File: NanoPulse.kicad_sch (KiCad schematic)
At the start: 0 parts

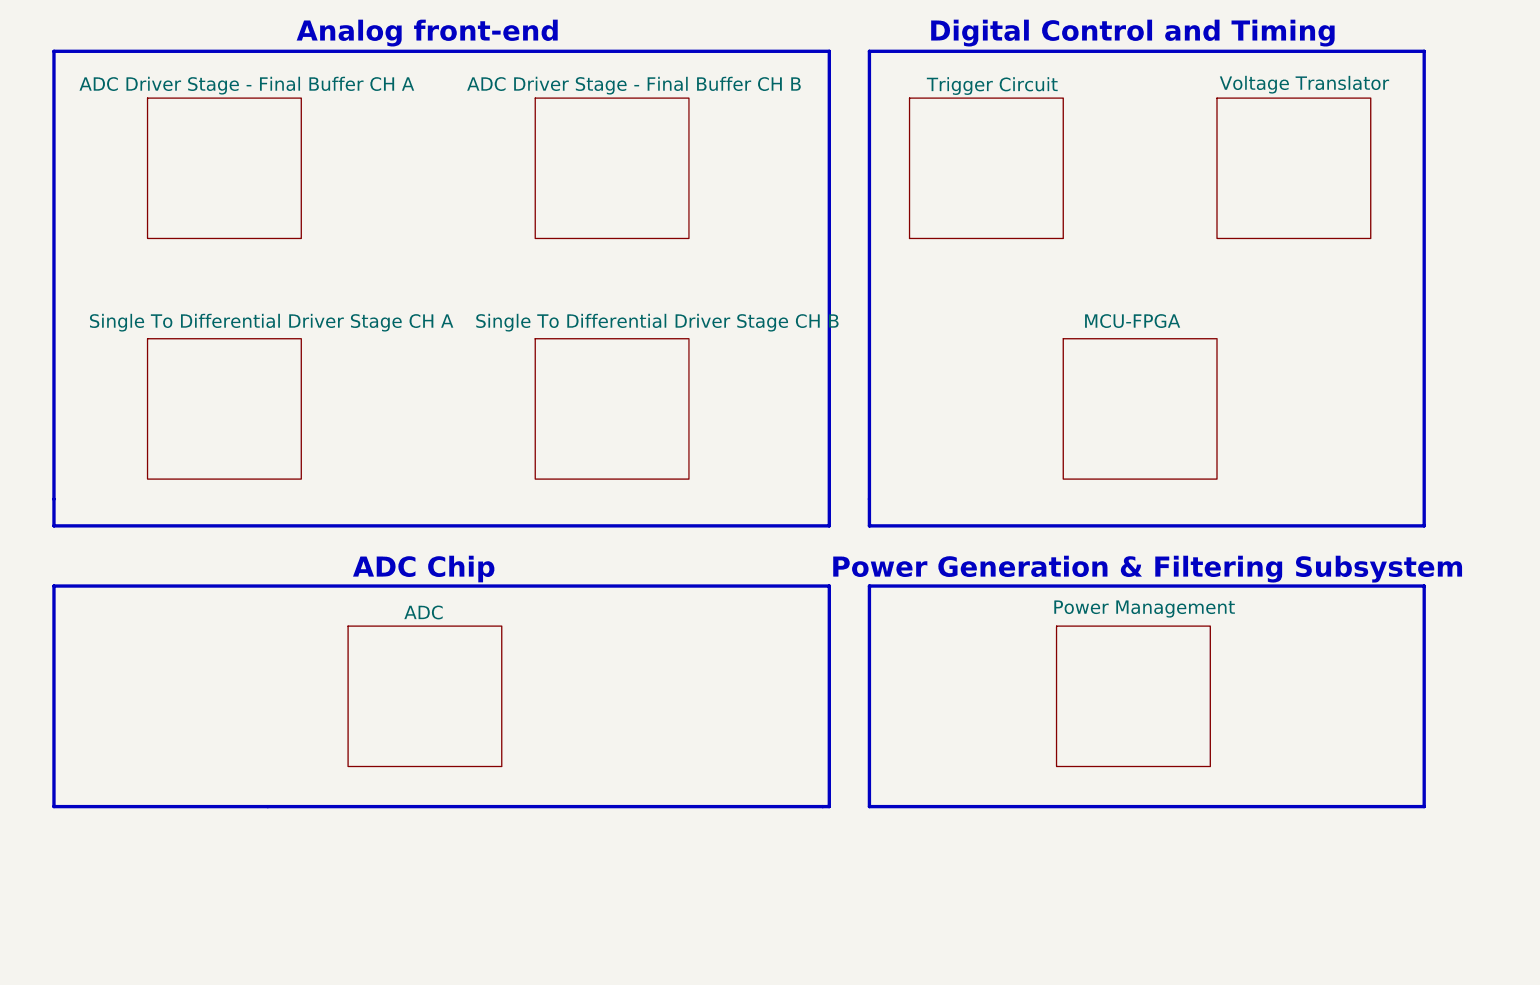
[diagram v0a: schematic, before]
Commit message: All done, Gerberd out :)
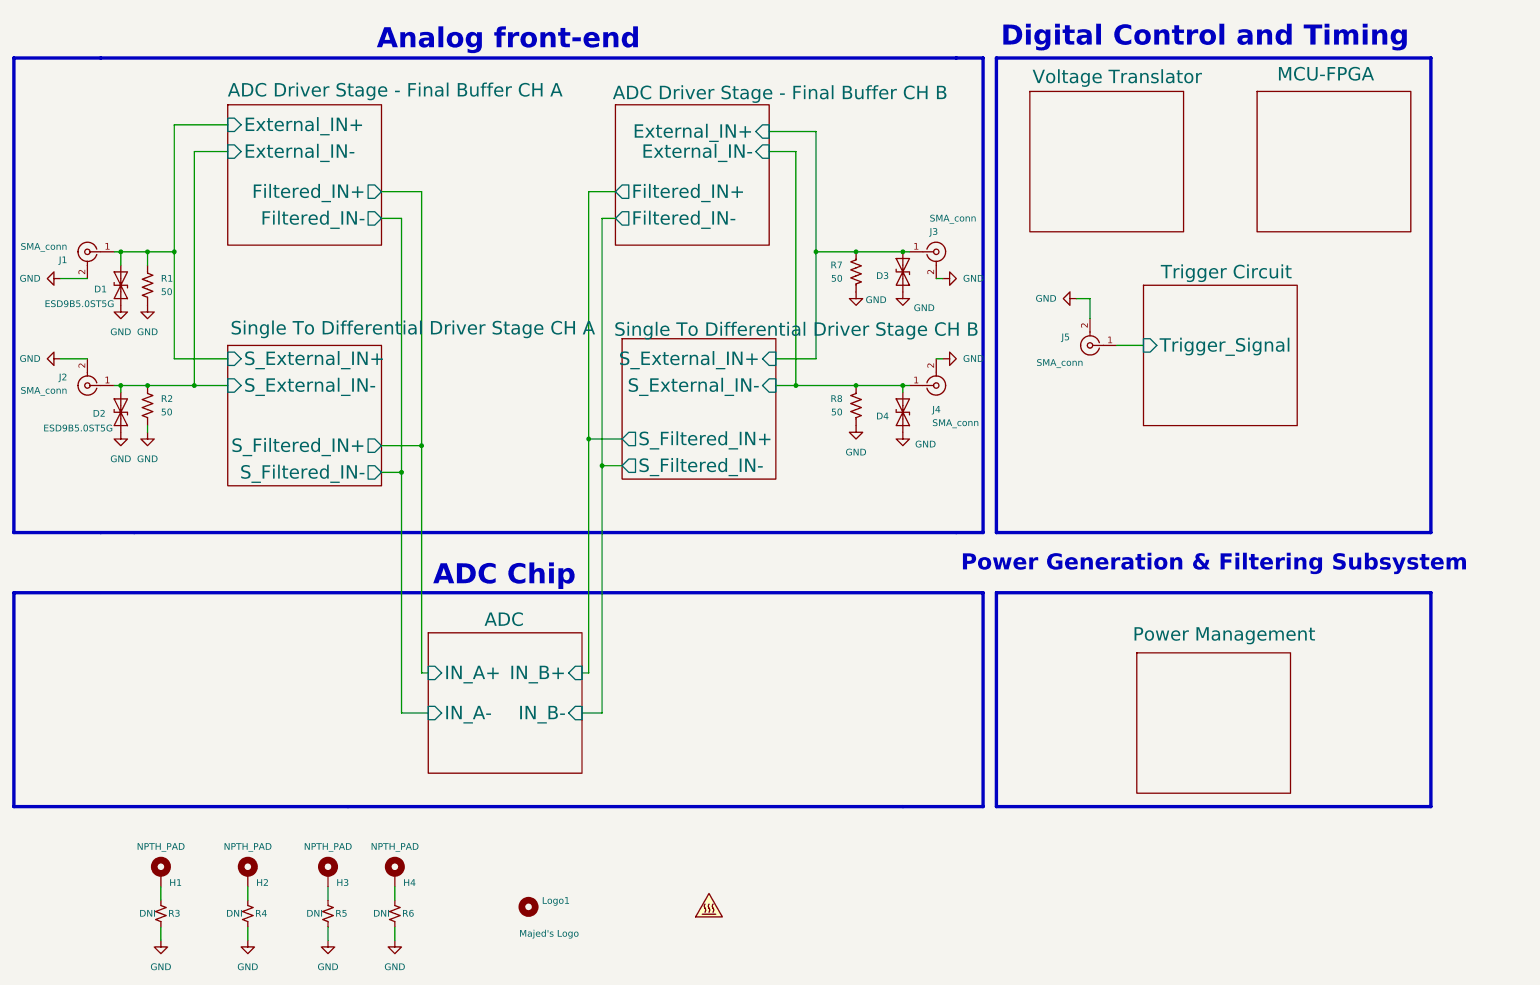
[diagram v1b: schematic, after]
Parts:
- added D1, D2, D3, D4: ESD9B5.0ST5G, Diode_SMD:D_SOD-923, symbol majed-symbols:ESD9B5.0ST5G
- added H1, H2, H3, H4: NPTH_PAD, Mounting_Wuerth:Mounting_Wuerth_WA-SMSI-M1.6_H3.5mm_ThreadDepth2mm_NoNPTH_97730356330, symbol majed-symbols:MountingHole_Pad_1
- added J1, J2, J3, J4, J5: SMA_conn, Connector_Coaxial:SMA_Amphenol_132289_EdgeMount, symbol majed-symbols:Conn_Coaxial
- added Logo1: Majed's Logo, Majed-footprints:Logo_Majed_small, symbol majed-symbols:MountingHole
- added R1, R2, R7, R8: 50, Resistor_SMD:R_0603_1608Metric, symbol majed-symbols:R_US
- added R3, R4, R5, R6: DNI, Resistor_SMD:R_0603_1608Metric, symbol majed-symbols:R_Small_US
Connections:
- new net: H2.1, R4.2
- new net: H3.1, R5.2
- new net: H4.1, R6.2
- new net: H1.1, R3.2
- new net ADC Driver Stage - Final Buffer CH A/External_IN+: D1.2 (A2), J1.1 (In), R1.1
- new net ADC Driver Stage - Final Buffer CH A/External_IN-: D2.2 (A2), J2.1 (In), R2.1
- new net ADC Driver Stage - Final Buffer CH B/External_IN+: D3.2 (A2), J3.1 (In), R7.1
- new net ADC Driver Stage - Final Buffer CH B/External_IN-: D4.2 (A2), J4.1 (In), R8.1
- new net GND: D1.1 (A1), D2.1 (A1), D3.1 (A1), D4.1 (A1), J1.2 (Ext), J2.2 (Ext), J3.2 (Ext), J4.2 (Ext), J5.2 (Ext), R1.2, R2.2, R3.1, R4.1, R5.1, R6.1, R7.2, R8.2
- new net Trigger Circuit/Trigger_Signal: J5.1 (In)
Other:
- sheet ADC ports: added IN_A+, IN_A-, IN_B+, IN_B-; removed none
- sheet ADC Driver Stage - Final Buffer CH A ports: added External_IN+, External_IN-, Filtered_IN+, Filtered_IN-; removed none
- sheet ADC Driver Stage - Final Buffer CH B ports: added External_IN+, External_IN-, Filtered_IN+, Filtered_IN-; removed none
- sheet Single To Differential Driver Stage CH A ports: added S_External_IN+, S_External_IN-, S_Filtered_IN+, S_Filtered_IN-; removed none
- sheet Single To Differential Driver Stage CH B ports: added S_External_IN+, S_External_IN-, S_Filtered_IN+, S_Filtered_IN-; removed none
- sheet Trigger Circuit ports: added Trigger_Signal; removed none
